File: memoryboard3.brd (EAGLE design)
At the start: 18.3 x 35.7 mm, 16 parts, among them IC1 SPI Memory, IC2 SPI Memory, IC3 SPI Memory, IC4 SPI Memory, IC5 SPI Memory, IC6 SPI Memory, IC7 74LCX126, IC8 74LCX138, T3.1 TEENSY_3.0_BASIC-PGM

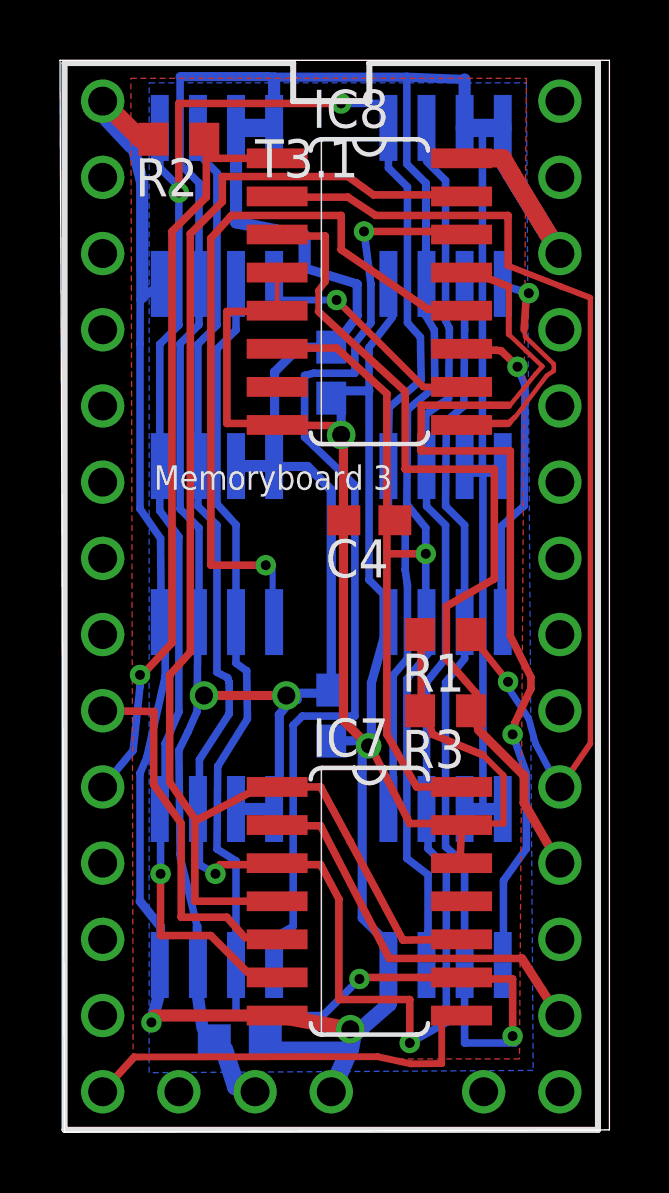
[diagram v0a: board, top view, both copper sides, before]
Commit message: update
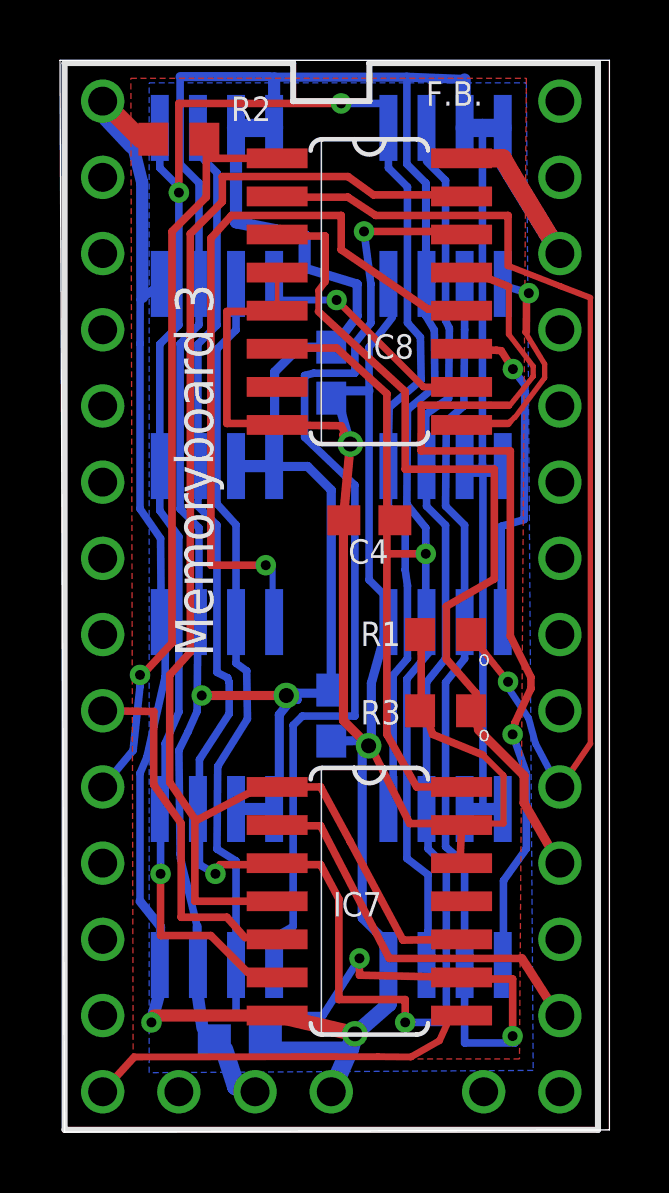
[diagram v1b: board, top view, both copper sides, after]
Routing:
- net SO: track 65.7 -> 66.7 mm
- net SO_T: track 14.1 -> 13.2 mm
- net SCK: track 71.5 -> 70.6 mm
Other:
- board text added: "1"
- board text added: "F.B."
- board text added: "o"
